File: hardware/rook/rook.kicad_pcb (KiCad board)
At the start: 2 copper layers, 77.9 x 50 mm, 29 parts, among them J1 Conn_01x02_Socket, J10 Micro_SD_Card, J2 Conn_01x04_Pin, J3 Conn_01x04_Pin, J4 Conn_01x01_Socket, J6 Conn_01x04_Socket, J7 Screw_Terminal_01x03, J8 Conn_01x03_Socket, J9 Conn_01x10_Socket, SW1 SW_Push, SW2 SW_Push, SW3 SW_Push, SW4 SW_Push, U1 wio-sx1262, U2 nice_nano_clean, U4 grove_a

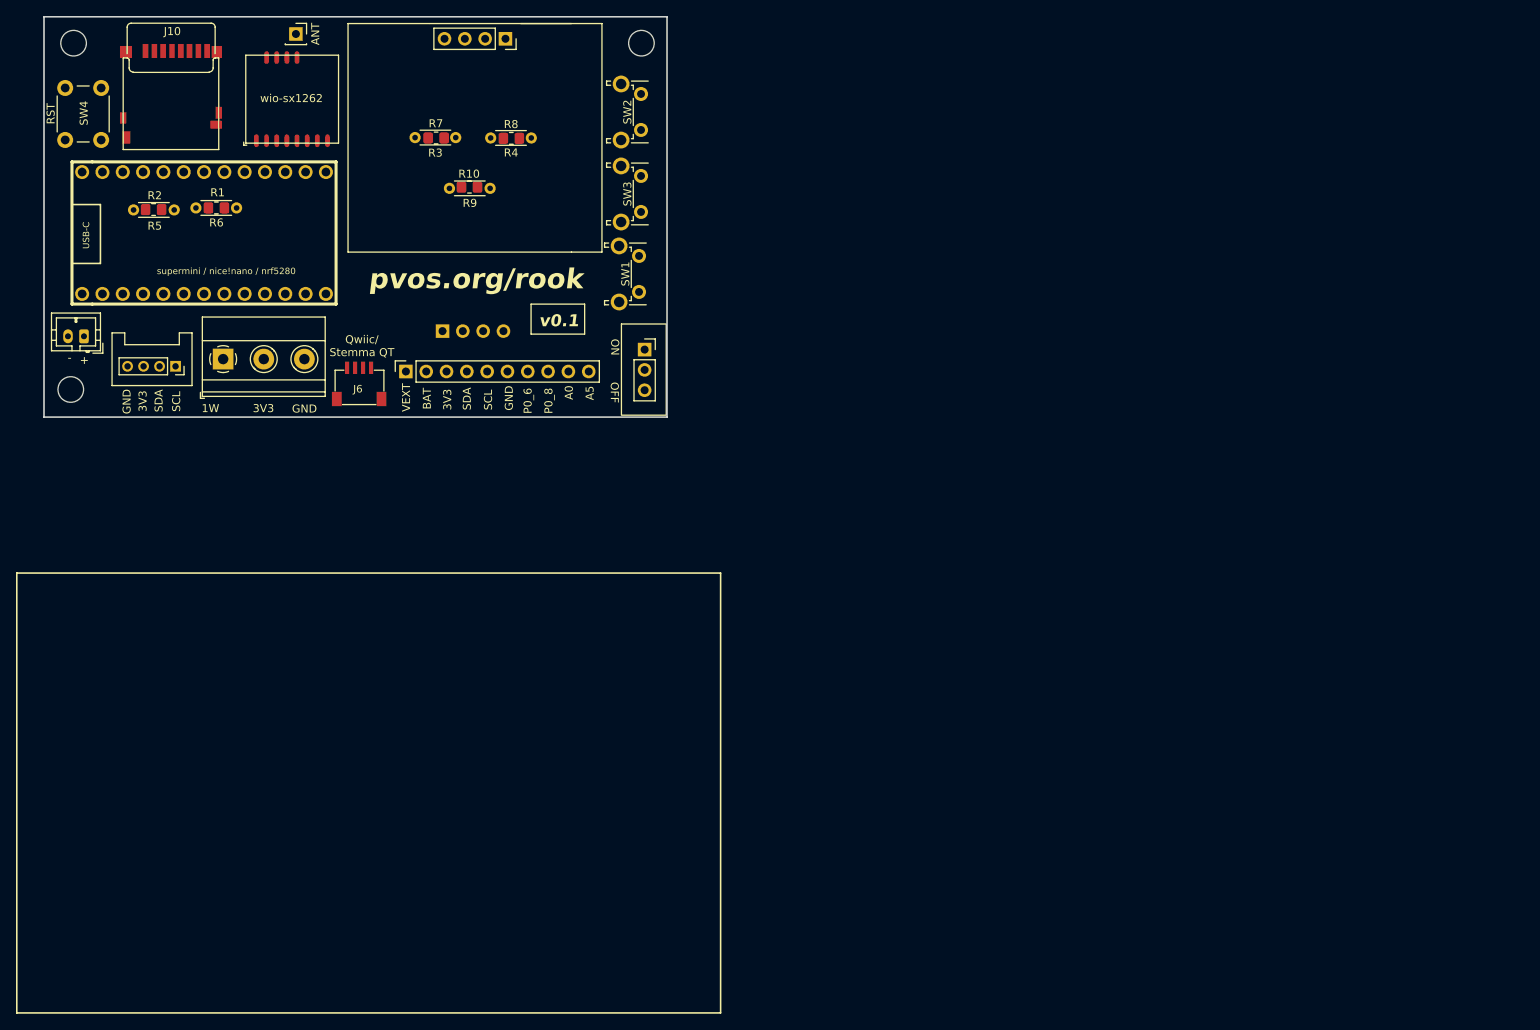
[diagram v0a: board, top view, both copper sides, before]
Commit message: update
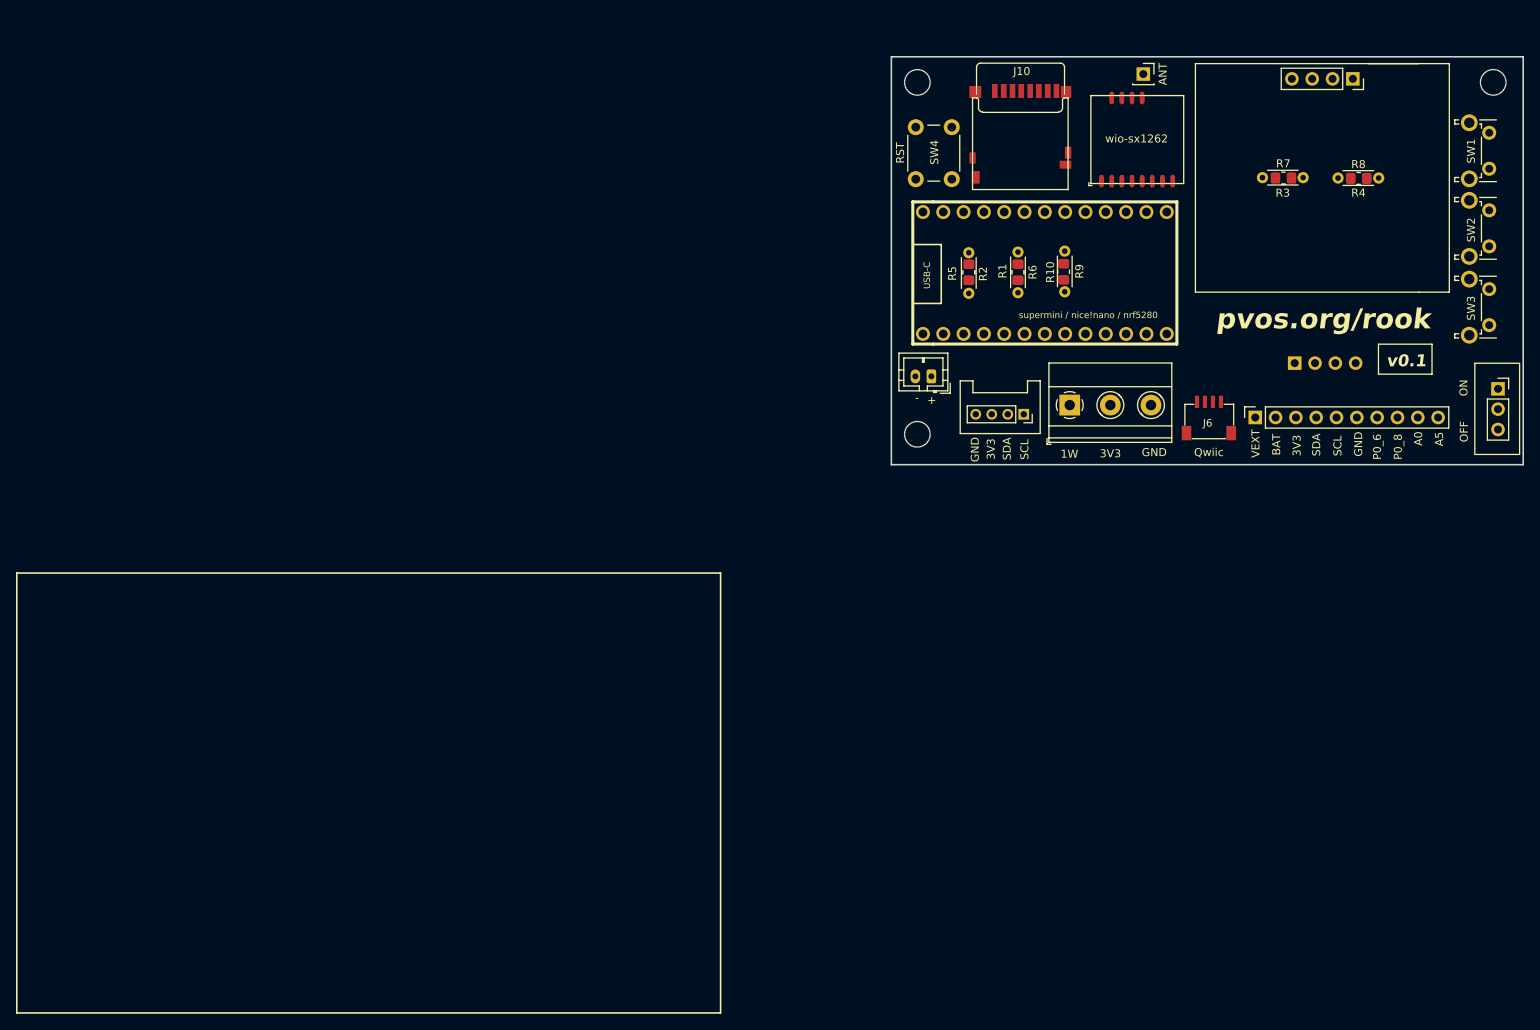
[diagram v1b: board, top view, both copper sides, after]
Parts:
- moved SW1 107.4 mm to (71.5, 6.30)
- moved SW2 107.0 mm to (71.5, 16.0)
- moved SW3 107.0 mm to (71.5, 25.9)
- moved J8 106.8 mm to (72.6, 38.3)
- moved J2 106.6 mm to (47.2, 35.1)
- moved H3 106.6 mm to (72.0, 0.00)
- moved SW4 106.5 mm to (4.30, 5.60)
- moved J9 106.4 mm to (42.2, 41.9)
- moved J6 106.3 mm to (36.5, 42.5)
- moved J10 106.3 mm to (12.9, 1.95)
- moved U4 106.2 mm to (13.3, 41.5)
- moved J1 106.1 mm to (1.75, 36.8)
- moved J3 106.1 mm to (54.5, -0.44)
- moved J4 106.1 mm to (28.2, -1.04)
- moved R4 106.1 mm to (57.7, 12.0)
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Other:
- board size 77.9 x 50 mm -> 79 x 51 mm
- board text added: "P0_20"
- board text added: "P0_22"
- board text added: "P1_06"
- board text added: "Qwiic"
- board text added: "RX"
- board text added: "TX"
- board text removed: "GPS_RX"
- board text removed: "GPS_TX"
- board text removed: "Qwiic/ Stemma QT"
